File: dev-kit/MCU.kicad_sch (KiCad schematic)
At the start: 38 parts, among them IC301 FAN5624UMPX, IC302 MX25U51245GZ4I00, IC303 USBLC6-2P6, IC304 NTS0104GU12, J301 Jumper, J302 Jumper, J303 Jumper, J304 Jumper, M301 NORA-B106, X301 Power, X302 Power, X303 Device, X304 GPIO, X305 UART, X306 IO Power, X307 Display, X308 Touch Power, X309 LED Power, X310 DEBUG

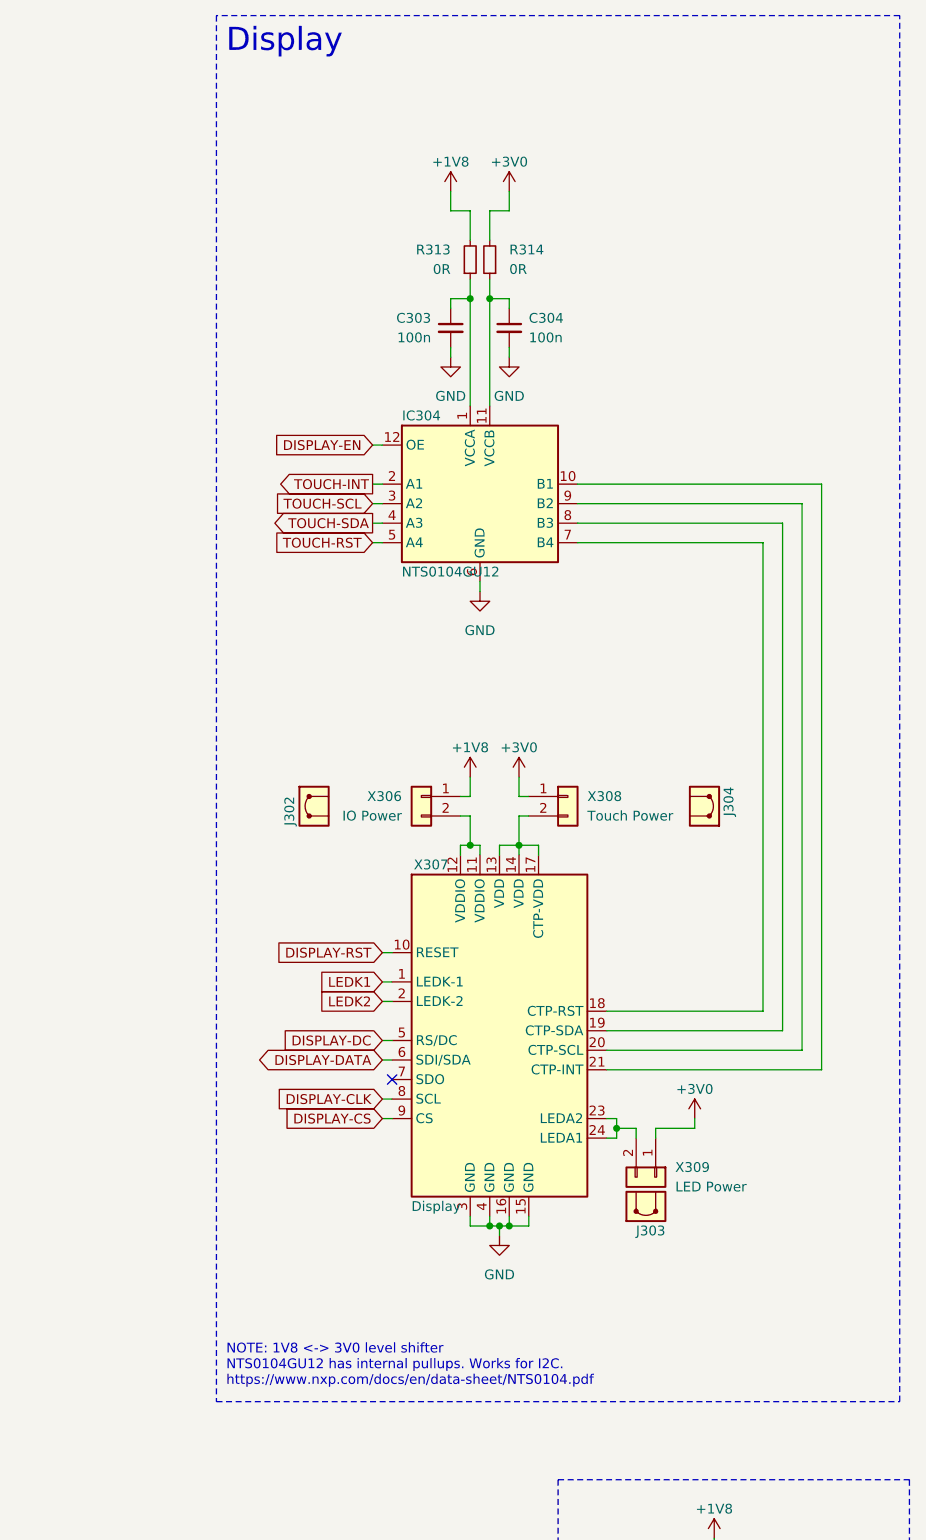
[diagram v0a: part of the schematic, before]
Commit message: Task: Issue #123
Signed-off-by: Daniel Kampert <DanielKampert@kampis-elektroecke.de>
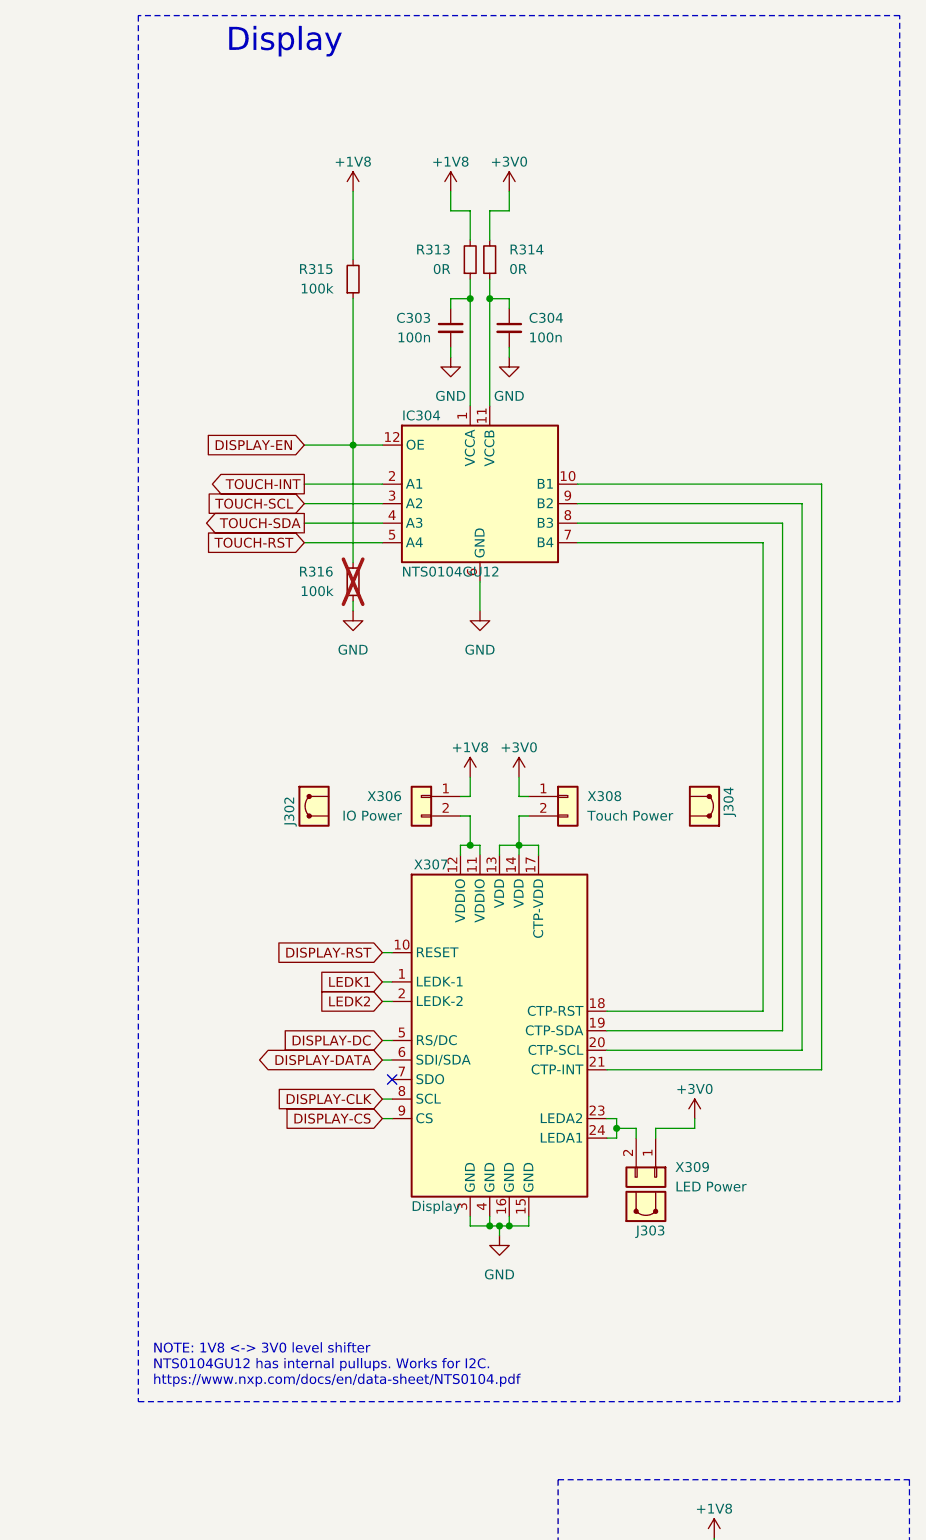
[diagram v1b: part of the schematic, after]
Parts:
- added R315, R316: 100k, Resistor_SMD:R_0805_2012Metric, symbol Device:R_Small
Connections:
- net +1V8: now also R315.2
- net DISPLAY-EN: now also R315.1, R316.2
- net GND: now also R316.1
